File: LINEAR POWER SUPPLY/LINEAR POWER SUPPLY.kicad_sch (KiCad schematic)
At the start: 11 parts, among them J1 SPADE, J2 SPADE, J3 SPADE, Q1 2SB817

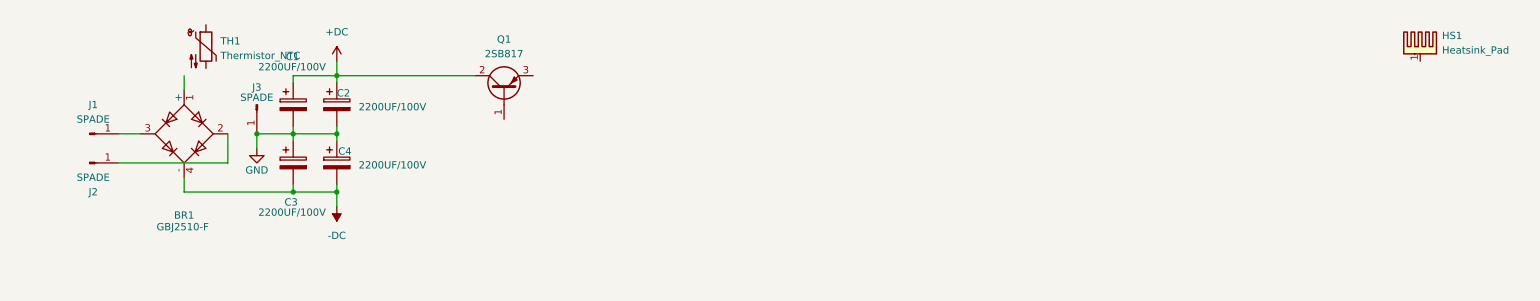
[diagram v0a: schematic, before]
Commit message: sdfasf
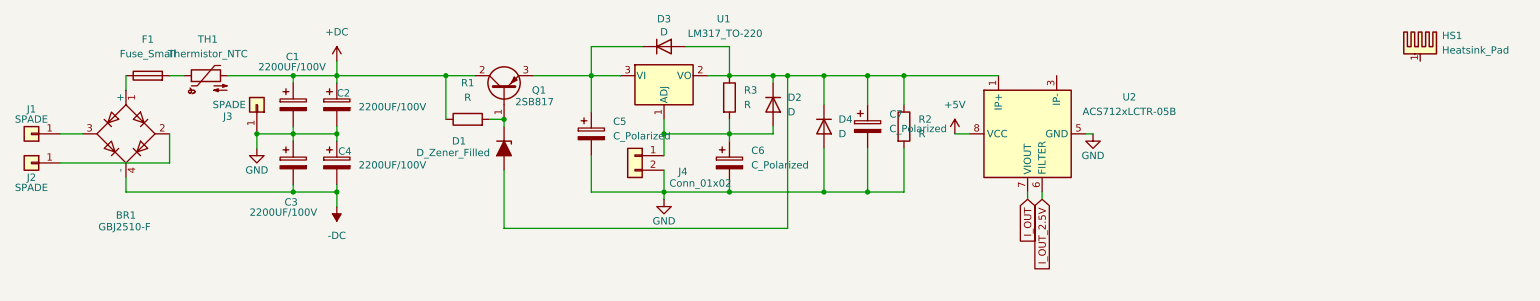
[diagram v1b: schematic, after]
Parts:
- added C5, C6, C7: C_Polarized, symbol Device:C_Polarized
- added D1: D_Zener_Filled, Diode_THT:D_DO-15_P5.08mm_Vertical_KathodeUp, symbol Device:D_Zener_Filled
- added D2, D3, D4: D, symbol Device:D
- added F1: Fuse_Small, Fuse:Fuseholder_Cylinder-5x20mm_Stelvio-Kontek_PTF78_Horizontal_Open, symbol Device:Fuse
- added J4: Conn_01x02, symbol Connector_Generic:Conn_01x02
- added R1: R, Resistor_THT:R_Axial_DIN0516_L15.5mm_D5.0mm_P7.62mm_Vertical, symbol Device:R
- added R2, R3: R, symbol Device:R
- added U1: LM317_TO-220, Package_TO_SOT_THT:TO-220-3_Vertical, symbol Regulator_Linear:LM317_TO-220
- added U2: ACS712xLCTR-05B, Package_SO:SOIC-8_3.9x4.9mm_P1.27mm, symbol Sensor_Current:ACS712xLCTR-05B
- J1, J2, J3: symbol Connector:Conn_01x01_Pin -> Connector_Generic:Conn_01x01
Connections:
- net +DC: now also TH1.2, R1.1
- net GND: now also C5.2, C6.2, C7.2, D4.2 (A), J4.2 (Pin_2), R2.2, U2.5 (GND)
- net at Q1.1 (B): now also D1.1 (K), R1.2
- net at Q1.3 (E): now also C5.1, D3.1 (K), U1.3 (VI)
- net at TH1.1: now also F1.2
- net at BR1.1 (+): now also F1.1
- new net: C7.1, D1.2 (A), D2.1 (K), D3.2 (A), D4.1 (K), R2.1, R3.1, U1.2 (VO), U2.1 (IP+), U2.2 (IP+)
- new net: C6.1, D2.2 (A), J4.1 (Pin_1), R3.2, U1.1 (ADJ)
- new net: U2.3 (IP-), U2.4 (IP-)
- new net +5V: U2.8 (VCC)
- new net I_OUT: U2.7 (VIOUT)
- new net I_OUT_2.5V: U2.6 (FILTER)
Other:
- moved on the sheet: BR1, J1, J2, J3, TH1
